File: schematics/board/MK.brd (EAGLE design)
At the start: 76 x 76 mm, 56 parts

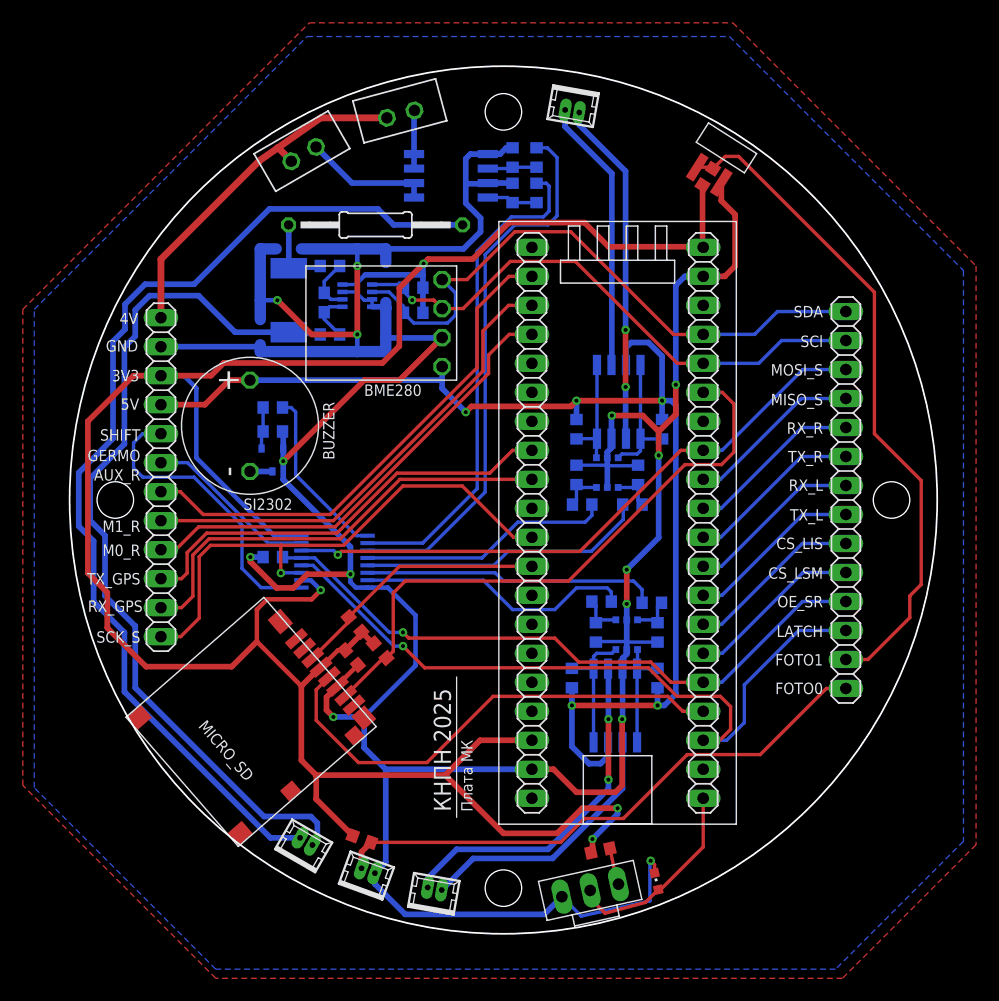
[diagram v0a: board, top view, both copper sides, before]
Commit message: СД в центре лепестка. Платы версия 2
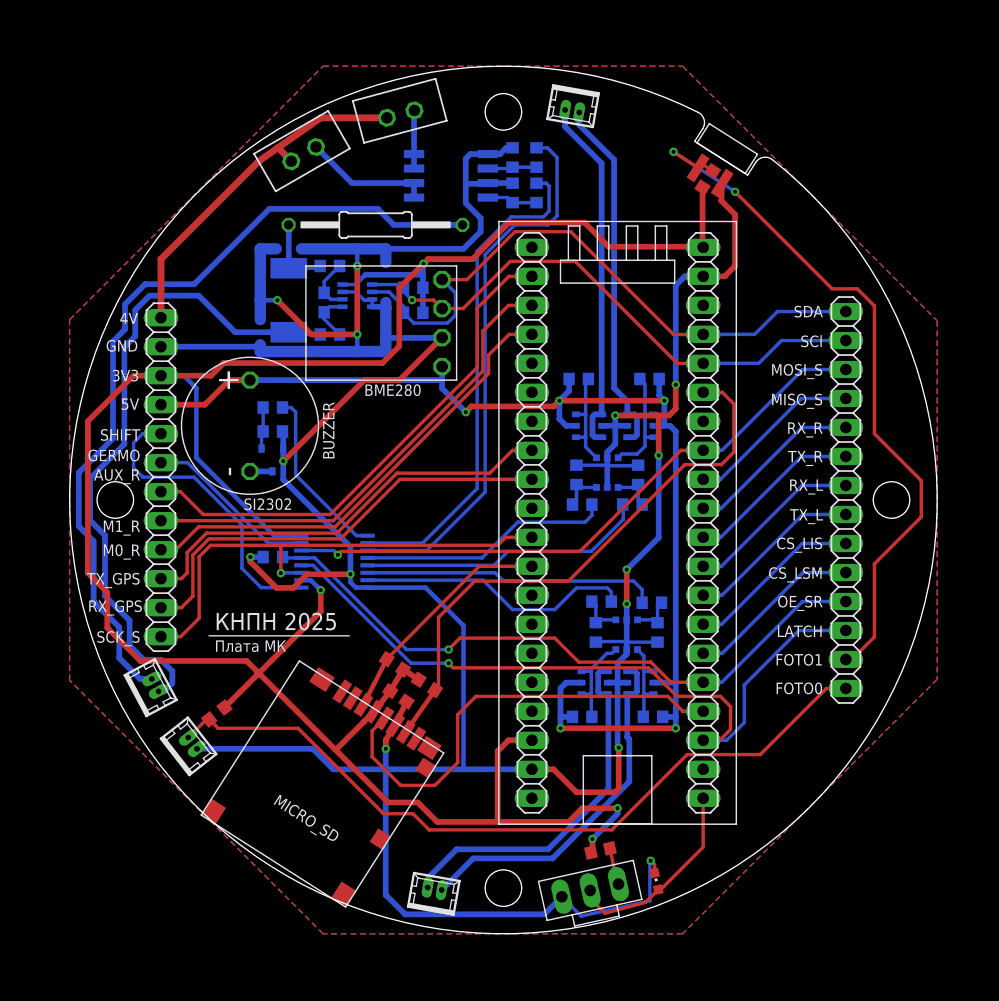
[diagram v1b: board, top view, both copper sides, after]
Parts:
- removed AP9930: MOSFET_2P+2N_AP9930GM, UNKNOWN-2024:SO8
- removed AP9930_: AP9930GM, UNKNOWN-2024:SO8
- added U$3, U$4, U$5, U$6: FDC6420C, KNPN-2023:TSOP-6
- moved U$1 26.9 mm to (14.2, 28.1), turned to 0 degrees
- moved SP 19.3 mm to (9.10, 23.6), turned to 298 degrees
- moved FOTO0 19.3 mm to (12.4, 18.4), turned to 308 degrees
- moved R7 16.8 mm to (14.9, 21.3), turned to 218 degrees
- moved MICRO_SD 10.8 mm to (26.2, 4.34), turned to 147.5 degrees
- moved C1 5.33 mm to (30.8, 22.8), turned to 147.5 degrees
- moved R5 5.08 mm to (33.3, 23.8), turned to 327.5 degrees
- moved R6 4.95 mm to (30.5, 25.6), turned to 147.5 degrees
- moved R32 4.54 mm to (52.8, 50.6), turned to 0 degrees
- moved R33 4.40 mm to (46.6, 50.6), turned to 180 degrees
- moved R26 3.52 mm to (46.9, 21.0), turned to 180 degrees
- moved R27 3.42 mm to (53.1, 21.0), turned to 0 degrees
- moved R0 0.20 mm to (57.9, 68.1)
- moved U$0 0.10 mm to (59.1, 69.9)
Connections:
- net 5V: now also U$3.P$2, U$4.P$2, U$5.P$2, U$6.P$2; no longer AP9930.7, AP9930_.7
- net GND: now also U$3.P$5, U$4.P$5, U$5.P$5, U$6.P$5; no longer AP9930.3, AP9930_.3
- net MOTOR1+: now also U$6.P$4, U$6.P$6; no longer AP9930.6
- net MOTOR1-: now also U$5.P$4, U$5.P$6; no longer AP9930.2
- net MOTOR2+: now also U$4.P$4, U$4.P$6; no longer AP9930_.6
- net MOTOR2-: now also U$3.P$4, U$3.P$6; no longer AP9930_.2
- net N$24: now also U$5.P$1, U$5.P$3; no longer AP9930.1, AP9930.8
- net N$25: now also U$3.P$1, U$3.P$3; no longer AP9930_.1, AP9930_.8
- net N$26: now also U$4.P$1, U$4.P$3; no longer AP9930_.4, AP9930_.5
- net N$27: now also U$6.P$1, U$6.P$3; no longer AP9930.4, AP9930.5
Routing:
- net SP-: track 91.6 -> 71.4 mm
- net SP+: track 77.5 -> 57.8 mm
- net GND: track 316.5 -> 335.5 mm
- net FOTO0: track 49.8 -> 67.4 mm
- net MOTOR2+: track 23.6 -> 31.6 mm
- net MOTOR1+: track 24.0 -> 31.5 mm
- net 3V3: track 221.7 -> 216.1 mm
- net FOTO1: track 58.7 -> 62.7 mm, vias 0 -> 2
- net SCK_SENS: track 47.2 -> 43.5 mm
- net D0_SD: track 53.2 -> 50.2 mm
- net N$25: track 11.7 -> 8.77 mm
- net 5V: track 108.7 -> 106.0 mm
- net CK_SD: track 42.7 -> 40.1 mm
- net CMD_SD: track 22.8 -> 20.6 mm
- net N$26: track 9.95 -> 7.85 mm
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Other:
- outline, holes or cut-outs redrawn
